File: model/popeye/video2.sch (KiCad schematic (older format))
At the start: 38 parts, among them U1 74LS10, U3 delay

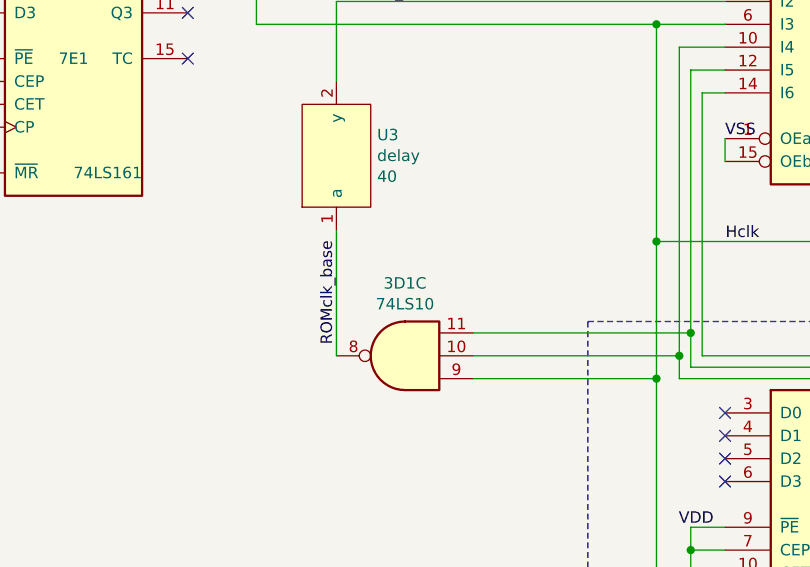
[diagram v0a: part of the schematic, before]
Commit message: Object test
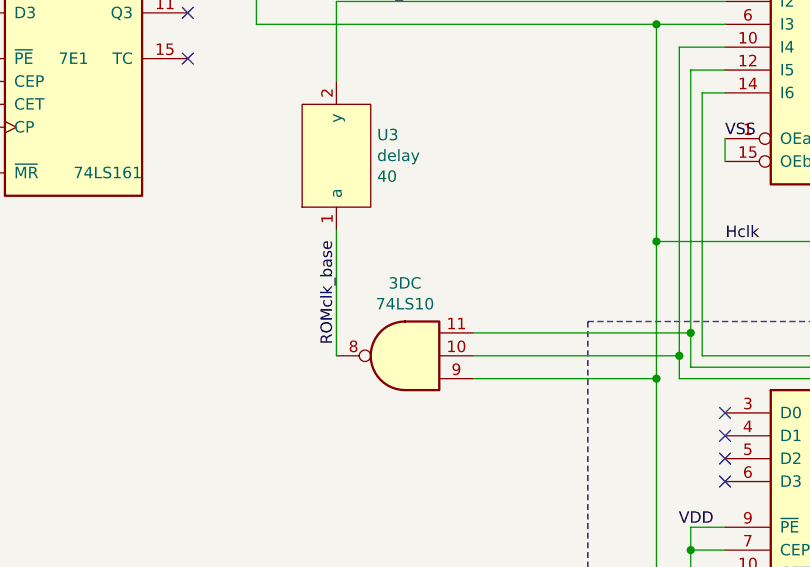
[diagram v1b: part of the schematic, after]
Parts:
- removed 3D1: 74LS10, symbol 74xx:74LS10
- added 3D: 74LS10, symbol jt74xx:74LS10
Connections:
- net Hclk: now also 3D.9
- net ROMclk_base: now also 3D.8
- net at 6D1.10 (I4), 6E1.14 (Q0): now also 3D.10
- net at 6D1.12 (I5), 6E1.13 (Q1): now also 3D.11
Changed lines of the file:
@@
 Text Label 2850 10550 3    50   ~ 0
 VSS
-$Comp
-L 74xx:74LS10 3D1
-U 3 1 5EAACC7A
-P 10800 9950
-F 0 "3D1" H 10800 9633 50  0000 C CNN
-F 1 "74LS10" H 10800 9724 50  0000 C CNN
-F 2 "" H 10800 9950 50  0001 C CNN
-F 3 "http://www.ti.com/lit/gpn/sn74LS10" H 10800 9950 50  0001 C CNN
-	3    10800 9950
-	-1   0    0    1
-$EndComp
 Wire Wire Line
 	11100 10050 11900 10050
@@
 Wire Wire Line
 	13400 5850 13200 5850
+$Comp
+L jt74xx:74LS10 3D
+U 3 1 5D2DE440
+P 10800 9950
+F 0 "3D" H 10800 9633 50  0000 C CNN
+F 1 "74LS10" H 10800 9724 50  0000 C CNN
+F 2 "" H 10800 9950 50  0001 C CNN
+F 3 "http://www.ti.com/lit/gpn/sn74LS10" H 10800 9950 50  0001 C CNN
+	3    10800 9950
+	-1   0    0    1
+$EndComp
 $EndSCHEMATC

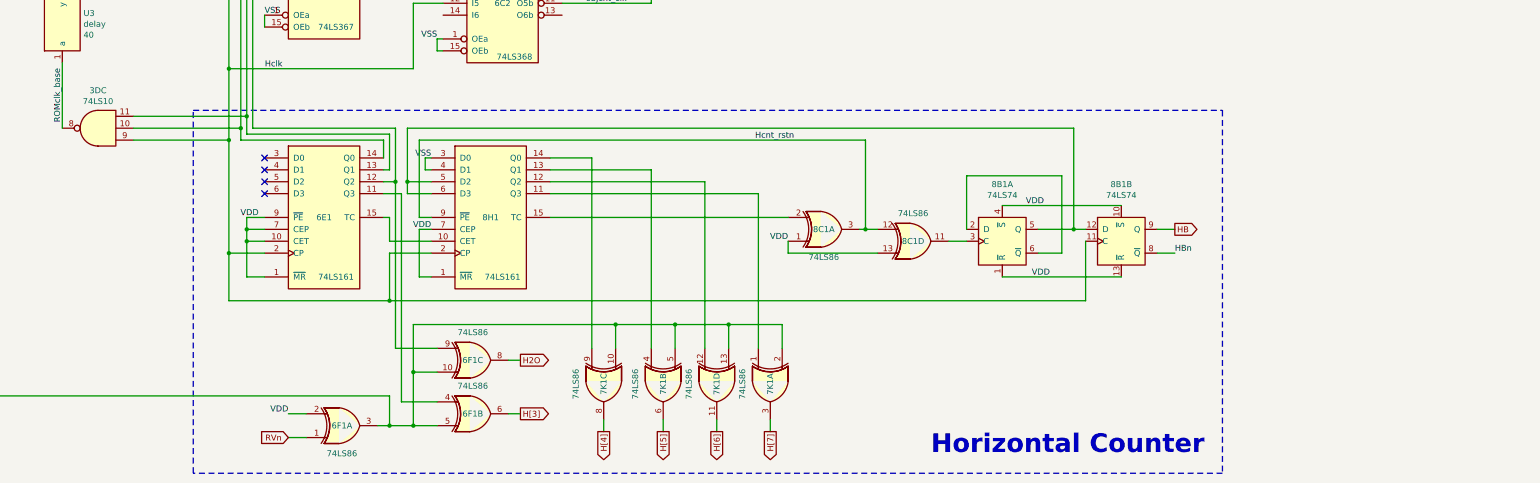
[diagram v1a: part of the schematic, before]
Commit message: Added HBDn to model
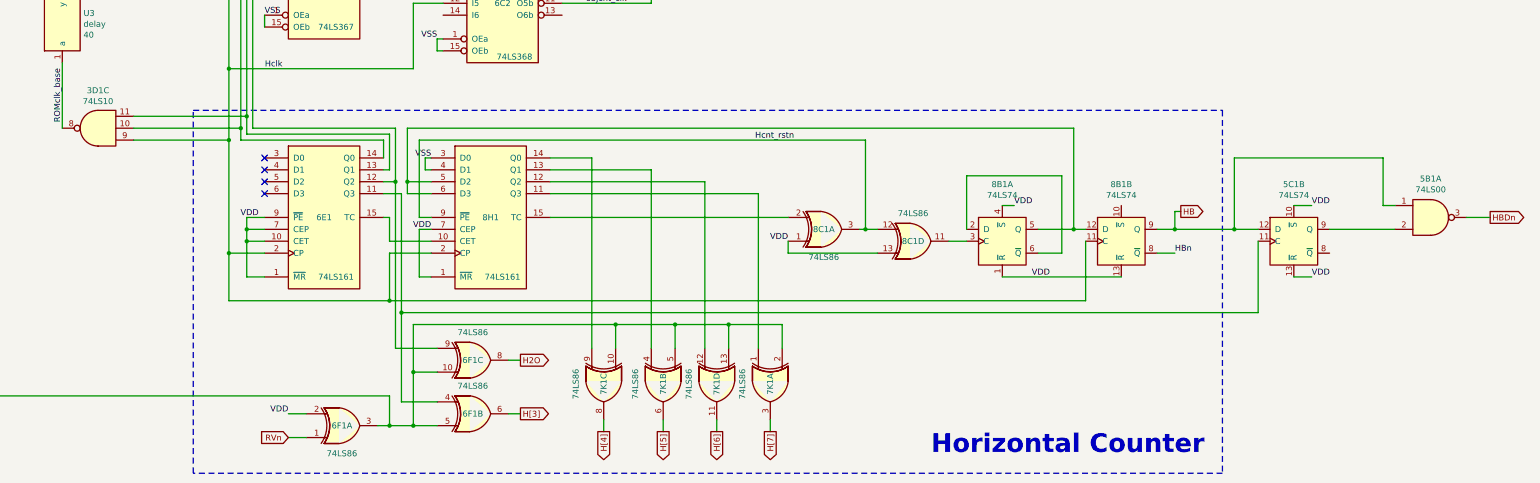
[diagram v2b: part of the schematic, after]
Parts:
- added 5B1: 74LS00, symbol jt74xx:74LS00
- added unit 2 of 5C1
- renumbered 3D to 3D1
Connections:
- net HB: now also 5B1.1, 5C1.12 (D)
- net VDD: now also 5C1.10 (~S), 5C1.13 (~R); no longer 8B1.10 (~S)
- net at 6E1.11 (Q3), 6F1.4: now also 5C1.11 (C)
- new net: 5B1.2, 5C1.9 (Q)
- new net HBDn: 5B1.3
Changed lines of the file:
@@
 	13200 10500 13350 10500
 Wire Wire Line
-	13350 10500 13350 12250
+	13350 10500 13350 11500
 Wire Wire Line
 	13350 12250 13650 12250
@@
 	19100 10800 19000 10800
 Wire Wire Line
-	19700 10800 19850 10800
-Wire Wire Line
 	19700 11000 19850 11000
-Text GLabel 19850 10800 2    50   Output ~ 0
+Text GLabel 19900 10650 2    50   Output ~ 0
 HB
 Text Label 19850 11000 0    50   ~ 0
 HBn
 Wire Wire Line
-	18400 11200 19400 11200
-Wire Wire Line
-	18400 10600 19400 10600
+	18400 10600 18500 10600
 Text Label 18800 11200 2    50   ~ 0
 VDD
-Text Label 18750 10600 2    50   ~ 0
+Text Label 18500 10600 0    50   ~ 0
 VDD
 Wire Wire Line
@@
 	13400 5850 13200 5850
 $Comp
-L jt74xx:74LS10 3D
+L jt74xx:74LS10 3D1
 U 3 1 5D2DE440
 P 10800 9950
-F 0 "3D" H 10800 9633 50  0000 C CNN
+F 0 "3D1" H 10800 9633 50  0000 C CNN
 F 1 "74LS10" H 10800 9724 50  0000 C CNN
 F 2 "" H 10800 9950 50  0001 C CNN
@@
 	-1   0    0    1
 $EndComp
+$Comp
+L jt74xx:74LS74 5C1
+U 2 1 5D4DDD61
+P 20850 10900
+F 0 "5C1" H 20850 11378 50  0000 C CNN
+F 1 "74LS74" H 20850 11287 50  0000 C CNN
+F 2 "" H 20850 10900 50  0001 C CNN
+F 3 "74xx/74hc_hct74.pdf" H 20850 10900 50  0001 C CNN
+	2    20850 10900
+	1    0    0    -1
+$EndComp
+$Comp
+L jt74xx:74LS00 5B1
+U 1 1 5D4DDF17
+P 22000 10700
+F 0 "5B1" H 22000 11025 50  0000 C CNN
+F 1 "74LS00" H 22000 10934 50  0000 C CNN
+F 2 "" H 22000 10700 50  0001 C CNN
+F 3 "http://www.ti.com/lit/gpn/sn74ls00" H 22000 10700 50  0001 C CNN
+	1    22000 10700
+	1    0    0    -1
+$EndComp
+Wire Wire Line
+	19700 10800 19850 10800
+Wire Wire Line
+	19900 10650 19850 10650
+Wire Wire Line
+	19850 10650 19850 10800
+Connection ~ 19850 10800
+Wire Wire Line
+	19850 10800 20350 10800
+Wire Wire Line
+	20350 10800 20350 10200
+Wire Wire Line
+	20350 10200 21600 10200
+Wire Wire Line
+	21600 10200 21600 10600
+Wire Wire Line
+	21600 10600 21700 10600
+Connection ~ 20350 10800
+Wire Wire Line
+	20350 10800 20550 10800
+Text GLabel 22500 10700 2    50   Output ~ 0
+HBDn
+Wire Wire Line
+	13350 11500 20550 11500
+Wire Wire Line
+	20550 11500 20550 10900
+Connection ~ 13350 11500
+Wire Wire Line
+	13350 11500 13350 12250
+Wire Wire Line
+	18400 11200 19400 11200
+Wire Wire Line
+	20850 10600 21000 10600
+Wire Wire Line
+	20850 11200 21000 11200
+Text Label 21000 10600 0    50   ~ 0
+VDD
+Text Label 21000 11200 0    50   ~ 0
+VDD
+Wire Wire Line
+	22300 10700 22500 10700
+Wire Wire Line
+	21150 10800 21700 10800
 $EndSCHEMATC
